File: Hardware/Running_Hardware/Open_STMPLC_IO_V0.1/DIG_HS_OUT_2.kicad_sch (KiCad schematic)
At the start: 24 parts, among them J13 Screw_Terminal_01x02, Q1 2N7002K, U14 TPS26600PWP, U15 NVTFS5124PLTAG

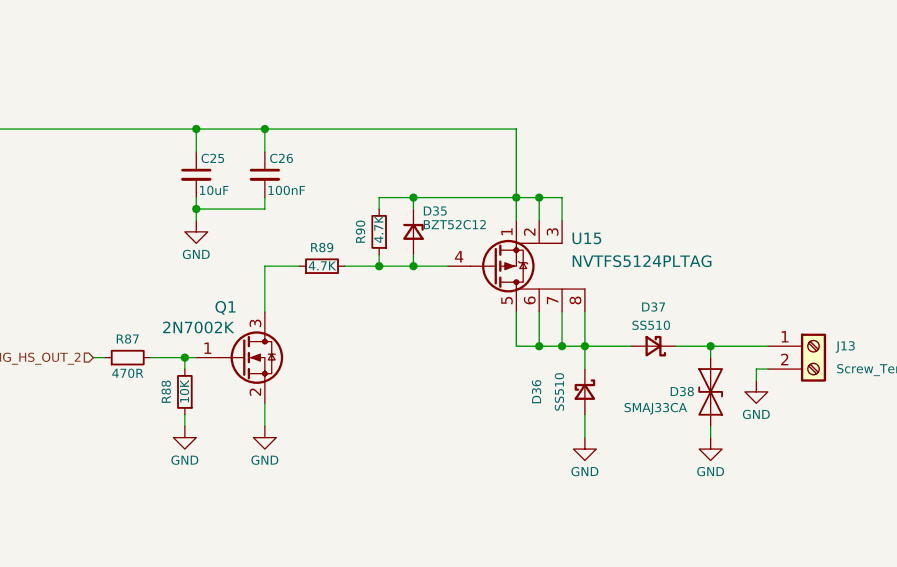
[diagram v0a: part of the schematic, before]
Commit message: Analog input section
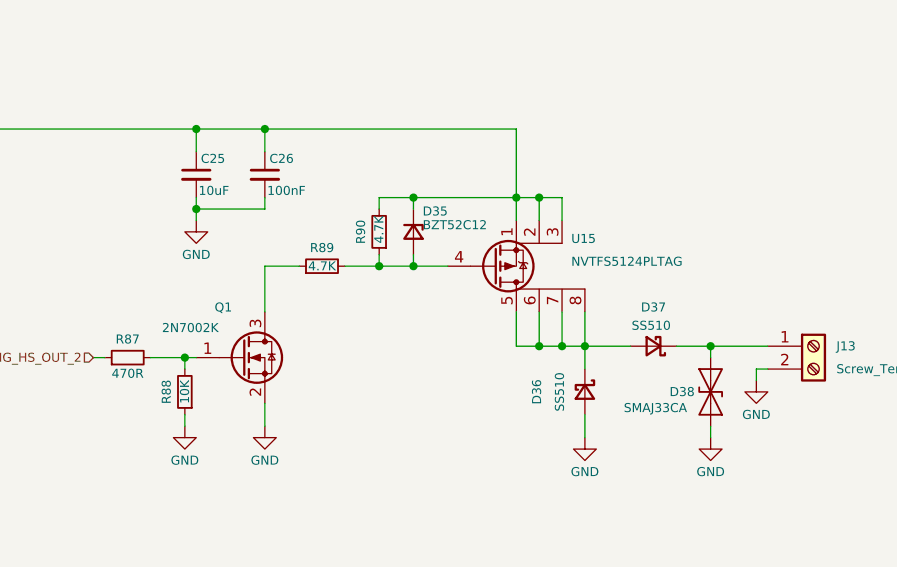
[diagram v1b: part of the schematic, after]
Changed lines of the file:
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@@
 			(effects
 				(font
-					(size 1.27 1.27)
+					(size 1 1)
 				)
 				(justify left)
@@
 			(effects
 				(font
-					(size 1.27 1.27)
+					(size 1 1)
 				)
 				(justify left)
@@
 			(effects
 				(font
-					(size 1.27 1.27)
+					(size 1 1)
 				)
 				(justify left)
@@
 			(effects
 				(font
-					(size 1.27 1.27)
+					(size 1 1)
 				)
 				(justify left)
